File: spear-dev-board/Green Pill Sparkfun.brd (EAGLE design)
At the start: 55 x 23 mm, 41 parts, among them IC1 STM32F103C8T6, IC2 STM32F103C8T6, U1 3.3V, X1 8MHz, X2 8MHz

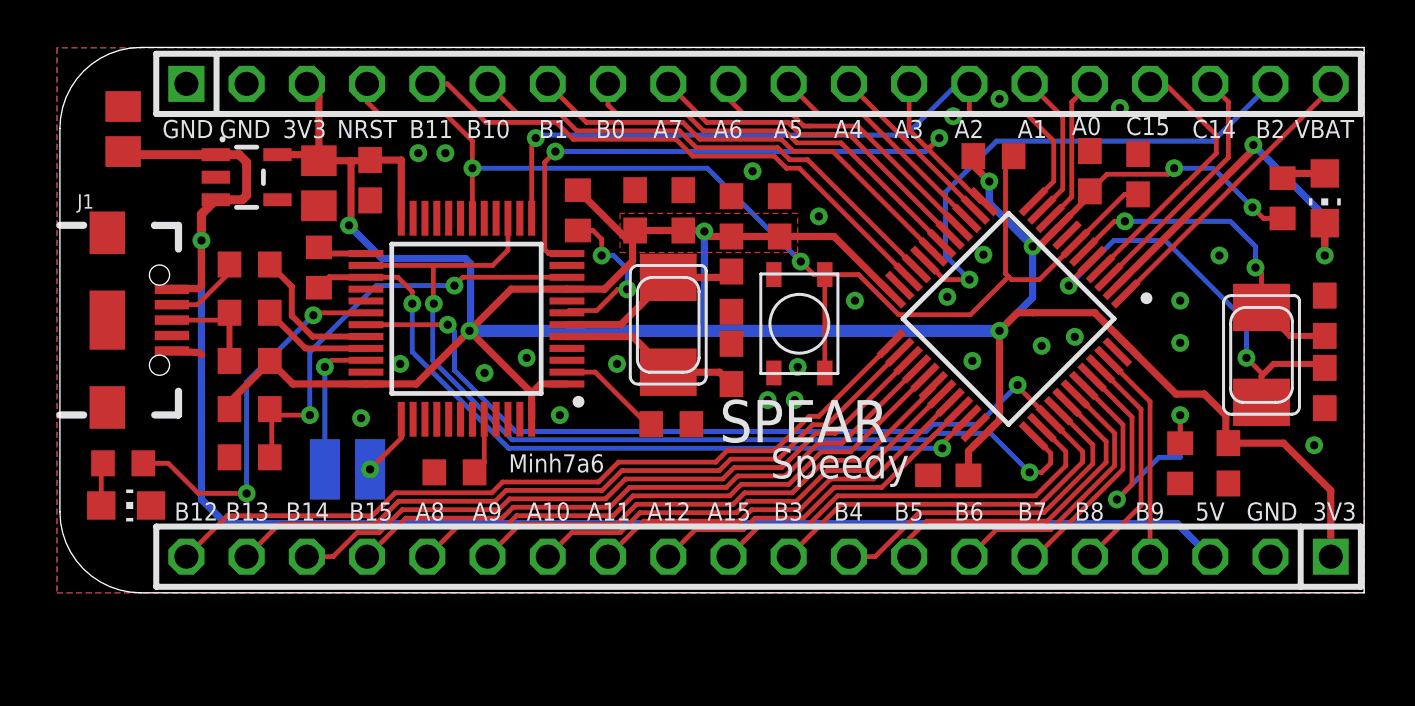
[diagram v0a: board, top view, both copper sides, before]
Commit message: uploaded bom, PnP, and change some board layout:
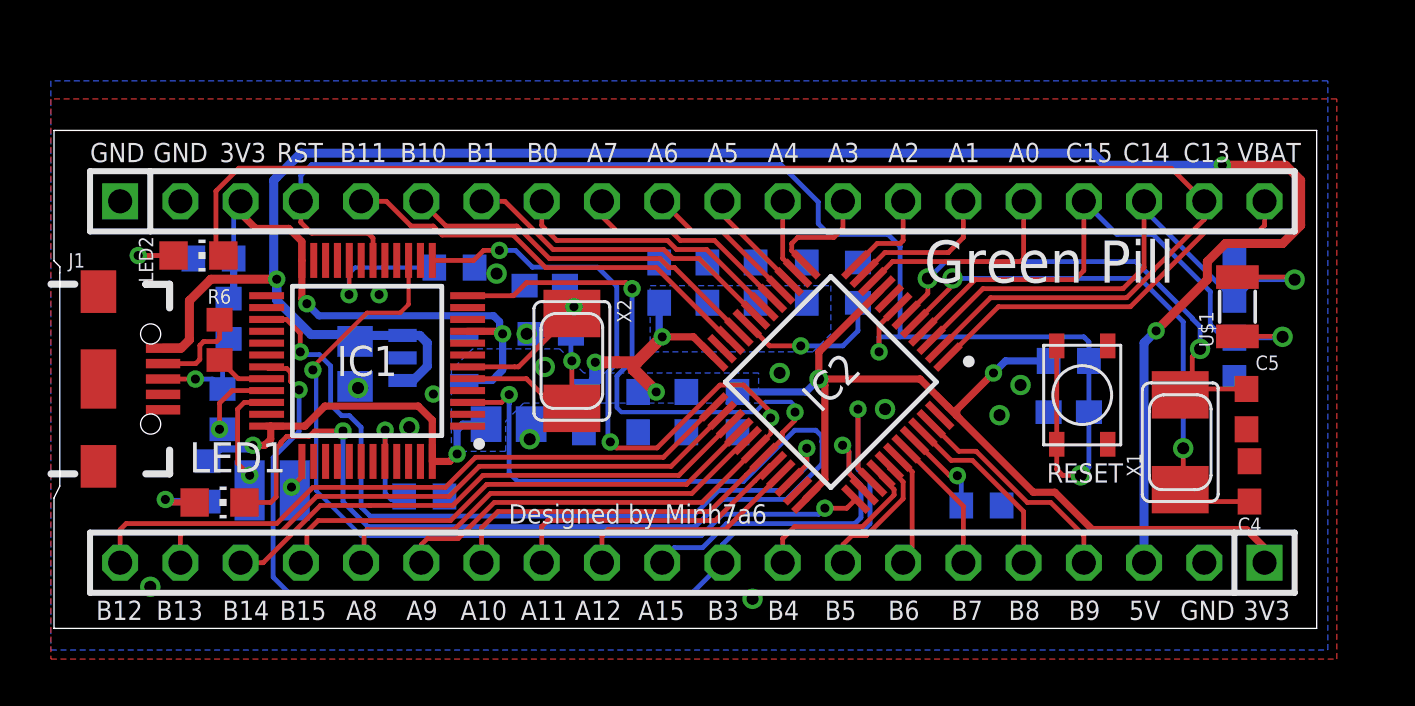
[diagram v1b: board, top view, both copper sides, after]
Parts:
- removed R11, R12: 4.7k, rcl:R0603
- removed R13: 1k, rcl:R0603
- added C6, C7: 22pF, resistor:C0603
- added U$1: 32.768kHz, SPEAR:3.2X1.5
- R1, R3: value 100k -> 10k
- R7: value 1.5k -> 10k
- R9: value 100 -> 1k
- moved LED2 47.6 mm to (5.84, 14.2), turned to 270 degrees
- moved R10 45.2 mm to (6.48, 14.1), flipped to the bottom, turned to 0 degrees
- moved C14 23.0 mm to (26.4, 7.62), flipped to the bottom
- moved C16 18.8 mm to (25.3, 13.1), flipped to the bottom
- moved C17 14.9 mm to (27.3, 13.1), flipped to the bottom, turned to 90 degrees
- moved C1 13.9 mm to (12.4, 9.65), flipped to the bottom, turned to 270 degrees
- moved C13 13.4 mm to (24.4, 7.62), flipped to the bottom, turned to 270 degrees
- moved C2 12.9 mm to (18.9, 7.11), flipped to the bottom, turned to 180 degrees
- moved U1 11.0 mm to (15.7, 9.91), flipped to the bottom, turned to 90 degrees
- moved C10 10.4 mm to (42.5, 7.62), flipped to the bottom, turned to 0 degrees
- moved R9 10.2 mm to (6.22, 4.70), flipped to the bottom, turned to 90 degrees
- moved R2 9.88 mm to (33.7, 13.1), flipped to the bottom, turned to 90 degrees
- moved U$2 9.85 mm to (42.0, 10.4), turned to 270 degrees
- moved R8 9.20 mm to (42.5, 9.78), flipped to the bottom, turned to 0 degrees
- moved C11 8.78 mm to (22.1, 7.62), flipped to the bottom, turned to 270 degrees
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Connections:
- removed net LED_STLINK: IC1.30, R13.1
- removed net PA0: IC1.10, R11.1, R12.2
- removed net RST: IC1.7, R4.1
- net 3.3V: now also R9.2; no longer IC1.1, R11.2, R4.2
- net GND: now also C6.2, C7.2, R4.2; no longer IC1.20, LED1.C, R12.1
- net N$5: now also IC1.20, R4.1; no longer IC1.2, R2.1
- net N$7: now also IC1.3, LED1.C; no longer LED1.A, R13.2
- net N$8: now also LED1.A; no longer IC1.25
- net OSC32_IN: now also C7.1, U$1.2
- net OSC32_OUT: now also C6.1, U$1.1
- net PA10: now also IC1.12
- net PA2: no longer IC1.13
- net PA3: no longer IC1.12
- net PA9: now also IC1.13
- net PB2: now also R2.1; no longer JP2.19
- net PC13: now also JP2.19
- net SWCLK: no longer IC1.26
- net SWDIO: no longer R9.2
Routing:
- net N$7: track 1.81 -> 52.1 mm, vias 0 -> 2
- net 3.3V: track 142.3 -> 93.2 mm, vias 8 -> 9
- net PC13: track 15.6 -> 59.8 mm, vias 2 -> 0
- net PA2: track 30.8 -> 4.07 mm, vias 1 -> 0
- net PA3: track 28.8 -> 4.71 mm, vias 2 -> 0
- net PA9: track 21.8 -> 42.1 mm, vias 0 -> 3
- net 5V: track 67.8 -> 87.2 mm, vias 1 -> 3
- net PA0: track 18.6 -> 0.00 mm, vias 2 -> 0
- net PA10: track 19.5 -> 37.7 mm, vias 0 -> 2
- net LED_STLINK: track 15.8 -> 0.00 mm, vias 2 -> 0
- net PB2: track 21.9 -> 6.51 mm
- net OSC32_IN: track 10.5 -> 24.1 mm, vias 0 -> 1
- net OSC32_OUT: track 11.4 -> 24.3 mm, vias 0 -> 1
- net NRST: track 51.4 -> 61.4 mm
- net BOOT0: track 12.5 -> 3.75 mm, vias 2 -> 1
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- added copper zone on layer 16, net 3.3V
- removed copper zone on layer 1, net 3.3V
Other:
- board size 55 x 23 mm -> 53.2 x 21 mm
- board text added: "C13"
- board text added: "Designed by Minh7a6"
- board text added: "Green Pill"
- board text added: "RESET"
- board text added: "RST"
- board text removed: "B2"
- board text removed: "Minh7a6"
- board text removed: "NRST"
- board text removed: "SPEAR"
- board text removed: "Speedy"
